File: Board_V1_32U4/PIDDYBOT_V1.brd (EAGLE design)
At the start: 48 x 76 mm, 49 parts, among them CN1 M02JST-PTH-2, CN2 M02JST-PTH-2, IC7 TLV71333DBV, U1 MPU-6050-1, U2 MCP73831, U3 ATMEGA328, U4 TB6621FNG, U5 BLUETOOTH-RN41, X1 Micro USB, Y1 8Mhz

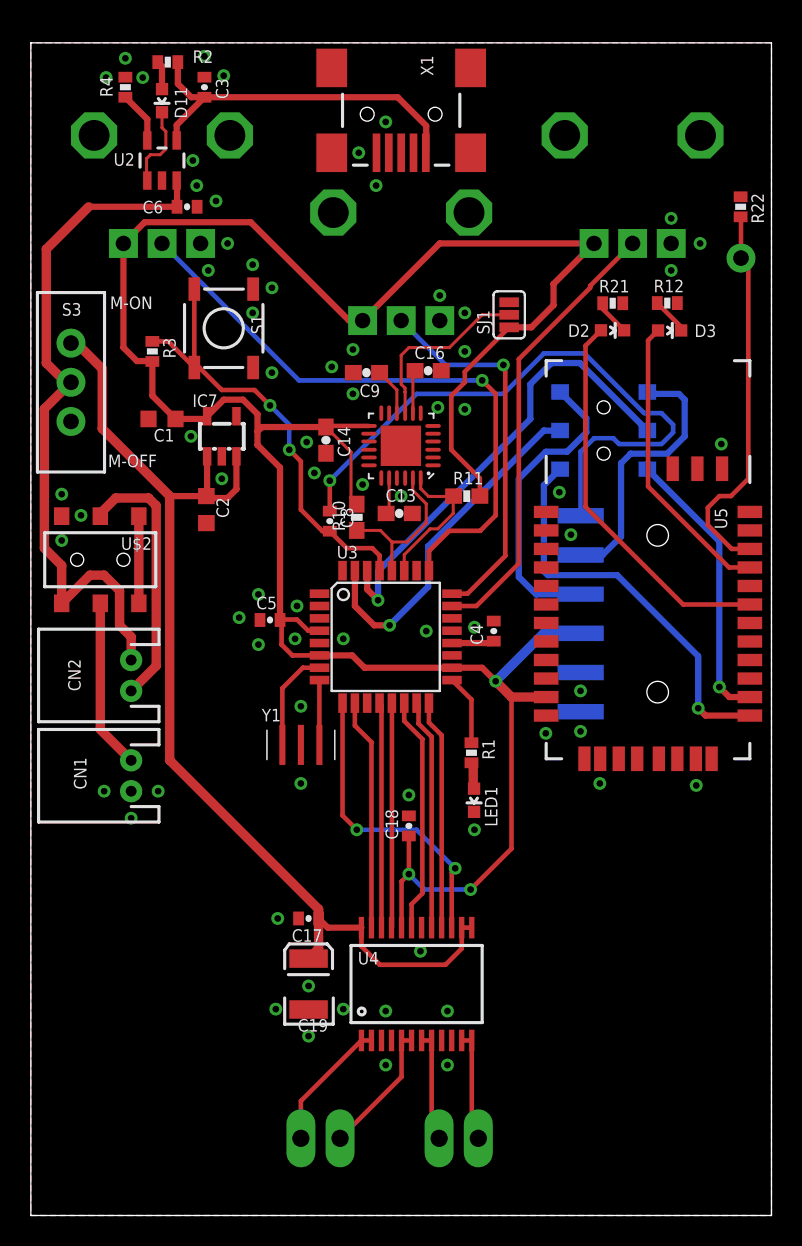
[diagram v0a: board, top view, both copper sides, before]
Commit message: Latest PIDDYBOT pcb finished ready to order
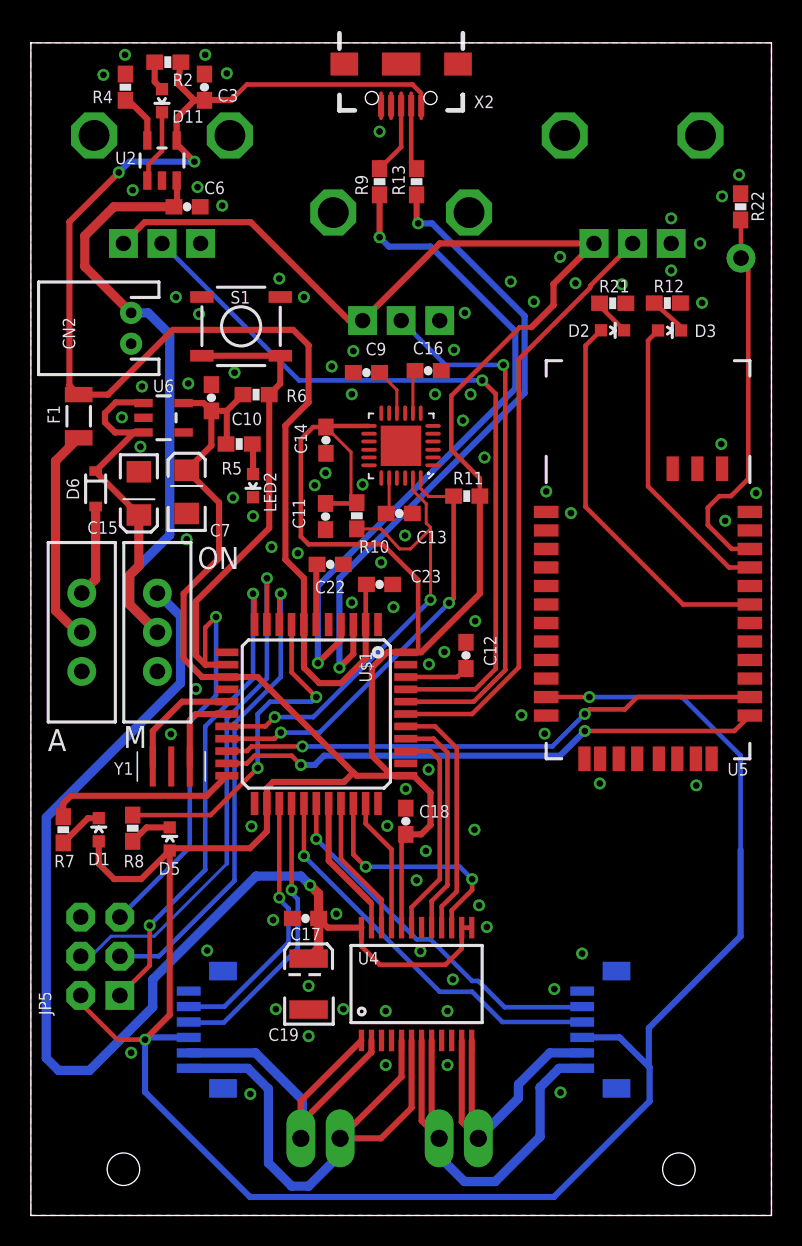
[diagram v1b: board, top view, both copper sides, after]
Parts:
- removed C1, C2: 100nF, rcl:C0603K
- removed C4, C5, C8: 0.1uF, SparkFun:0402-CAP
- removed CN1: M02JST-PTH-2, SparkFun-Connectors:JST-2-PTH
- removed IC7: TLV71333DBV, anoven:SOT-23-5
- removed JP1: (no value), SparkFun-Connectors:1X06-SMD
- removed LED1: BLUE, SparkFun:LED-0603
- removed R1: 1k, SparkFun:0402-RES
- removed R3: 10k, SparkFun:0402-RES
- removed SJ1: (no value), SparkFun:SJ_3_PASTE2&3
- removed U$2, U$3: AYZ0202, SparkFun-Electromechanical:AYZ0202
- removed U3: ATMEGA328, SparkFun:TQFP32-08
- removed X1: Micro USB, SparkFun:USB-MINIB
- added C10, C22, C23: 1uF, SparkFun:0603-CAP
- added C11, C12: 0.1uF, SparkFun:0603-CAP
- added C15, C7: 10uF, SparkFun:EIA3216
- added D1: Green, SparkFun:LED-0603
- added D5: Yellow, SparkFun:LED-0603
- added D6: (no value), SparkFun:SOD-323
- added F1: 500mA, SparkFun:PTC-1206
- added JP3, JP4: (no value), SparkFun-Connectors:1X06-1MM
- added JP5: (no value), SparkFun-Connectors:2X3-NS
- added LED2: Red, SparkFun:LED-0603
- added R13, R9: 22, SparkFun:0603-RES
- added R5: 1K, SparkFun:0603-RES
- added R6: 10K, SparkFun:0603-RES
- added R7, R8: 330, SparkFun:0603-RES
- added S2: (no value), SparkFun-Electromechanical:SWITCH-SPDT
- added U$1: ATMEGA32U4TQFP, SparkFun-DigitalIC:SPARKFUN-DIGITALIC_TQFP44
- added U6: MIC5219, SparkFun:SOT23-5
- added X2: (no value), Testing:USB-AB-MICRO-SMD-V03-IN&OUT
- C17, C18, C3, C6: device SparkFun:0402-CAP -> SparkFun:0603-CAP
- R12, R2, R21, R22, R4: device SparkFun:0402-RES -> SparkFun:0603-RES
- moved CN2 22.5 mm to (6.50, 57.5)
- moved S3 16.2 mm to (3.30, 37.8)
- moved Y1 8.52 mm to (9.10, 29.1), turned to 180 degrees
- moved S1 1.13 mm to (13.6, 57.6), turned to 0 degrees
- moved C18 0.36 mm to (24.3, 25.6)
- moved C17 0.20 mm to (17.8, 19.2)
- moved R10 0.10 mm to (21.1, 45.4)
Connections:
- removed net AD3: U3.26
- removed net ADO: SJ1.2, U1.9
- removed net BT-RXI: U$3.3, U5.13
- removed net BT-TXO: U$3.6, U5.14
- removed net CHARGE: C6.1, CN2.2, S3.2, U$2.4, U2.3
- removed net DTR: C8.1, JP1.1
- removed net IO2: U3.32
- removed net IO4: U3.2
- removed net IO7: U3.11
- removed net N$10: U$2.3, U$2.6
- removed net N$5: U3.8, Y1.3
- removed net N$8: CN1.2, U$2.5
- removed net PROG-RXI: JP1.2, U$3.4
- removed net PROG-TXO: JP1.3, U$3.1
- removed net VCC: C1.1, C14.1, C18.1, C5.2, IC7.5, JP1.4, R10.2, R11.2, R3.2, SJ1.1, U$16.P$3, U$17.P$3, U$18.P$3, U1.13, U3.18, U3.4, U3.6, U4.20, U5.11
- removed net VIN: C3.1, R2.2, U2.4, X1.VBUS
- new net 3.3V: C10.1, C11.2, C14.1, C18.1, C7.A, D1.A, D5.A, JP3.4, JP4.4, JP5.2, R10.2, R11.2, R5.2, R6.2, U$1.14, U$1.24, U$1.34, U$1.44, U$16.P$3, U$17.P$3, U$18.P$3, U1.13, U4.20, U5.11, U6.5
- new net D+: R9.1, U$1.4
- new net D-: R13.1, U$1.3
- new net D11: U$1.12
- new net D14: R8.1, U$1.8
- new net D7: U$1.1
- new net MISO: JP5.1, U$1.11
- new net MOSI: JP5.4, U$1.10
- new net MTE_A_1: JP3.2, U$1.25
- new net MTE_A_2: JP3.3, U$1.26
- new net MTE_B_1: JP4.3, U$1.27
- new net MTE_B_2: JP4.2, U$1.28
- new net N$1: U$1.17, Y1.1
- new net N$15: C22.2, U$1.6
- new net N$16: R13.2, X2.D-1
- new net N$17: R9.2, X2.D+1
- new net N$19: D5.C, R8.2
- new net N$20: D1.C, R7.2
- new net N$38: LED2.A, R5.1
- new net TXLED: R7.1, U$1.22
- new net UVCC: C23.2, C3.1, F1.1, R2.2, U$1.2, U$1.7, U2.4, X2.VBUS1
- new net V_MOTOR: C17.1, C19.A, S2.3, U4.13, U4.14, U4.24
- net A01: now also JP3.5
- net A02: now also JP3.6
- net AIN1: now also U$1.32; no longer U3.13
- net AIN2: now also U$1.30; no longer U3.12
- net AREF: now also C12.2, U$1.42; no longer C4.1, U3.20
- net B01: now also JP4.5
- net B02: now also JP4.6
- net BIN1: now also U$1.37; no longer U3.15
- net BIN2: now also U$1.38; no longer U3.16
- net GND: now also C10.2, C11.1, C12.1, C15.C, C22.1, C23.1, C7.C, CN2.1, JP3.1, JP4.1, JP5.6, LED2.C, U$1.15, U$1.23, U$1.33, U$1.35, U$1.43, U$1.5, U1.9, U6.2, X2.GND1; no longer C1.2, C2.2, C4.2, C5.1, CN1.1, IC7.2, JP1.6, LED1.C, SJ1.3, U$2.1, U3.21, U3.3, U3.5, X1.GND
- net N$2: now also U$1.16, Y1.3; no longer CN2.1, U$2.2
- net N$3: now also F1.2, S3.2; no longer LED1.A, R1.2
- net N$4: now also D6.2, S3.3; no longer U3.7, Y1.1
- net POTD: now also U$1.41; no longer U3.25
- net POTI: now also U$1.40; no longer U3.24
- net POTP: now also U$1.39; no longer U3.23
- net PWMA: now also U$1.29; no longer U3.10
- net PWMB: now also U$1.31; no longer U3.9
- net RESET: now also JP5.5, R6.1, U$1.13; no longer C8.2, R3.1, U3.29
- net RX-I: now also U$1.20, U5.14; no longer U$3.5, U3.30
- net SCK: now also JP5.3, U$1.9; no longer R1.1, U3.17
- net SCL: now also U$1.18; no longer U3.28
- net SDA: now also U$1.19; no longer U3.27
- net STBY: now also U$1.36; no longer U3.14
- net TX-O: now also U$1.21, U5.13; no longer U$3.2, U3.31
- net V_BATT: now also C15.A, C6.1, CN2.2, D6.1, S2.2, U2.3, U6.1, U6.3; no longer C17.1, C19.A, C2.1, IC7.1, IC7.3, S3.3, U4.13, U4.14, U4.24
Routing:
- net 3.3V: track 0.00 -> 298.3 mm, vias 0 -> 2
- net VCC: track 158.3 -> 0.00 mm, vias 3 -> 0
- net UVCC: track 0.00 -> 93.3 mm, vias 0 -> 2
- net V_MOTOR: track 0.00 -> 77.2 mm, vias 0 -> 1
- net CHARGE: track 46.1 -> 0.00 mm
- net D+: track 0.00 -> 44.0 mm, vias 0 -> 2
- net D-: track 0.00 -> 42.2 mm, vias 0 -> 2
- net DTR: track 41.0 -> 0.00 mm, vias 1 -> 0
- net MOSI: track 0.00 -> 34.5 mm, vias 0 -> 1
- net MISO: track 0.00 -> 31.7 mm, vias 0 -> 2
- net A02: track 8.64 -> 35.5 mm
- net SCK: track 4.58 -> 31.3 mm, vias 0 -> 1
- net BT-RXI: track 26.3 -> 0.00 mm, vias 1 -> 0
- net MTE_B_1: track 0.00 -> 25.9 mm, vias 0 -> 1
- net RESET: track 29.3 -> 54.4 mm, vias 2 -> 1
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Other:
- board text added: "A"
- board text added: "D"
- board text added: "I"
- board text added: "Idlehandsdevelopment.com"
- board text added: "M"
- board text added: "ON"
- board text added: "P"
- board text added: "PIDDYBOT_V4"
- board text removed: "M-OFF"
- board text removed: "M-ON"
